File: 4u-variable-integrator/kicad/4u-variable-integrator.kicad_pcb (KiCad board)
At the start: 2 copper layers, 99.1 x 152.4 mm, 91 parts, among them J1 Banana Socket PanelMount, J10 Banana Socket PanelMount, J11 Banana Socket PanelMount, J12 Conn_01x04_Female, J13 Conn_01x04_Male, J14 Conn_01x02_Female, J15 Conn_01x02_Male, J16 Banana Socket PanelMount, J17 4U_Power, J18 Banana Socket PanelMount, J19 Banana Socket PanelMount, J2 Banana Socket PanelMount, J20 Conn_01x04_Female, J21 Conn_01x04_Male, J22 Banana Socket PanelMount, J23 Banana Socket PanelMount, J3 Banana Socket PanelMount, J4 Conn_01x04_Female, J5 Conn_01x04_Female, J6 Conn_01x04_Male, J7 Conn_01x04_Male, J8 Banana Socket PanelMount, J9 Banana Socket PanelMount, Q1 2N3906, Q2 2N3906, U1 TL074, U2 LM13700, U4 TL072

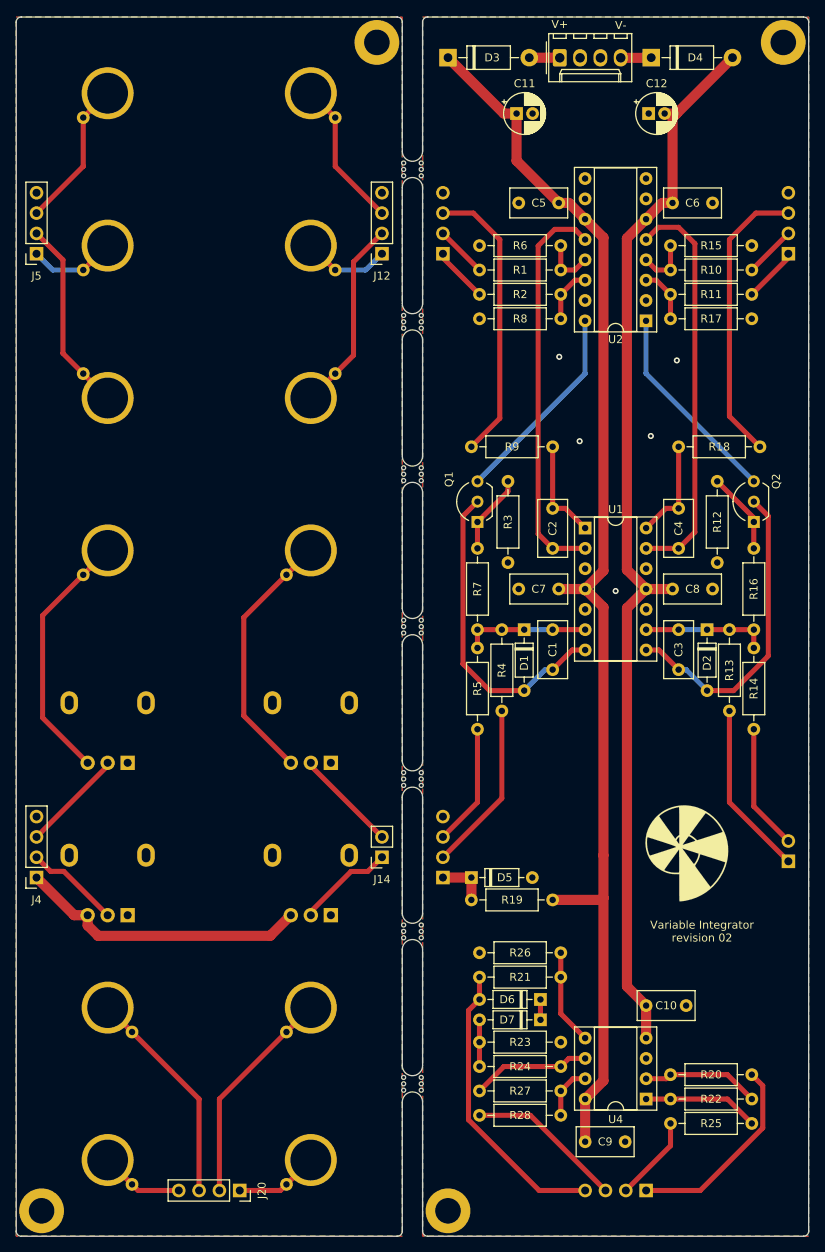
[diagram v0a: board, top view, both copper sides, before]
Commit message: Refreshing kicad projects
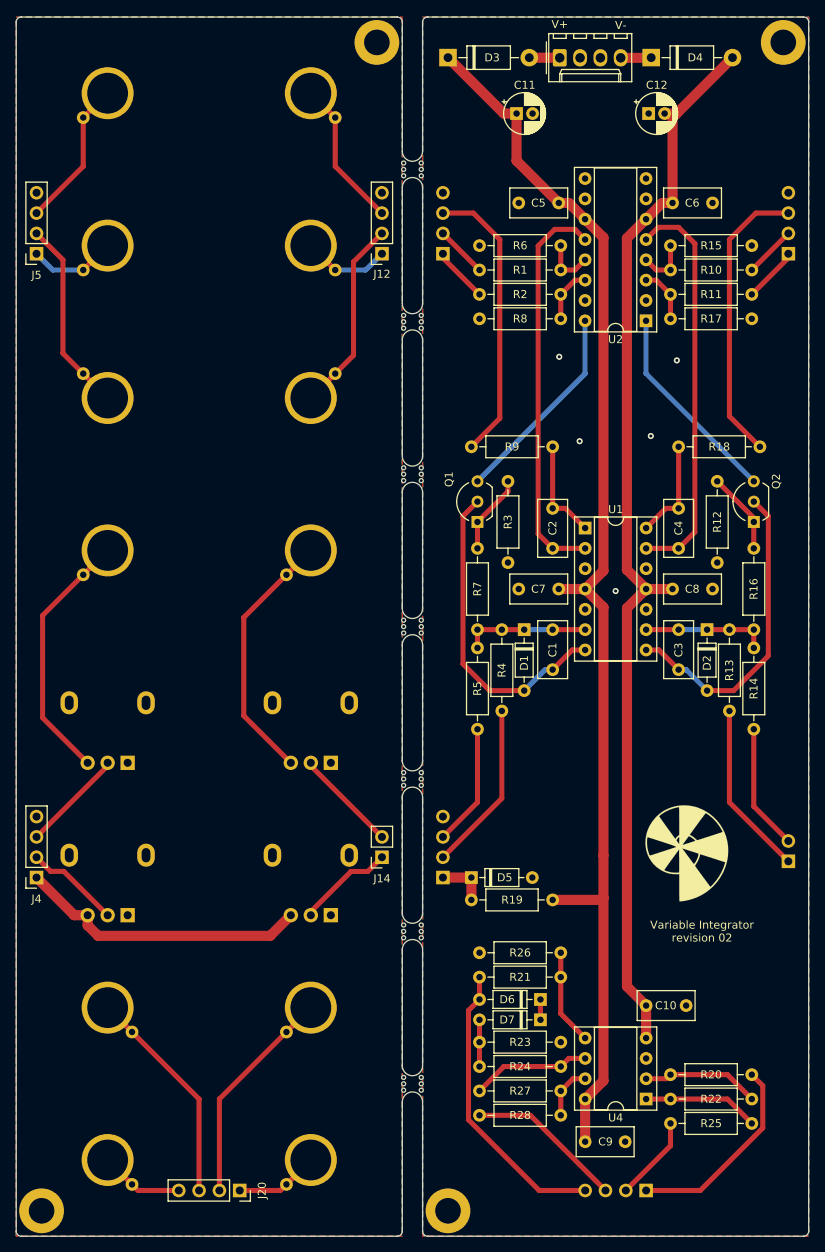
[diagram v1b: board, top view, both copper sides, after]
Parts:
- C1, C10, C2, C3, C4, C5, C6, C7, C8, C9: footprint rumblesan-standard-parts:C_Rect_L7.0mm_W3.5mm_P5.00mm -> Rumblesan_Standard_Parts:C_Rect_L7.0mm_W3.5mm_P5.00mm
- C11, C12: value 1uF -> 10uF; footprint rumblesan-standard-parts:CP_Radial_D5.0mm_P2.00mm -> Rumblesan_Standard_Parts:CP_Radial_D5.0mm_P2.00mm
- D1, D2: value 1n4148 -> 1N4148; footprint rumblesan-standard-parts:D_DO-35_SOD27_P7.62mm_Horizontal -> Rumblesan_Standard_Parts:D_DO-35_SOD27_P7.62mm_Horizontal
- D3, D4: footprint rumblesan-standard-parts:D_DO-41_SOD81_P10.16mm_Horizontal -> Rumblesan_Standard_Parts:D_DO-41_SOD81_P10.16mm_Horizontal
- D5, D6, D7: footprint rumblesan-standard-parts:D_DO-35_SOD27_P7.62mm_Horizontal -> Rumblesan_Standard_Parts:D_DO-35_SOD27_P7.62mm_Horizontal
- H1, H2, H3, H4: footprint rumblesan-standard-parts:MountingHole_3.2mm_M3_DIN965_Pad -> Rumblesan_Standard_Parts:MountingHole_3.2mm_M3_DIN965_Pad
- J1, J10, J11, J16, J18, J19, J2, J22, J23, J3, J8, J9: footprint rumblesan-standard-parts:BananaJack_THT_JohnsonCinch_108-09 -> Rumblesan_Standard_Parts:BananaJack_THT_JohnsonCinch_108-09
- J17: footprint 4u-power:4u_Power_Molex_KK-254_P2.54mm -> 4U_Power:4u_Power_Molex_KK-254_P2.54mm
- R1, R10, R11, R12, R13, R14, R15, R16, R17, R18, R19, R2, R20, R21, R22, R23, R24, R25, R26, R27, R28, R3, R4, R5, R6, R7, R8, R9: footprint rumblesan-standard-parts:R_Axial_DIN0207_L6.3mm_D2.5mm_P10.16mm_Horizontal -> Rumblesan_Standard_Parts:R_Axial_DIN0207_L6.3mm_D2.5mm_P10.16mm_Horizontal
- RV1, RV2, RV3, RV4: footprint rumblesan-standard-parts:Potentiometer_Alpha_RD901F-40-00D_Single_Vertical -> Rumblesan_Standard_Parts:Potentiometer_Alpha_RD901F-40-00D_Single_Vertical
- U1: footprint rumblesan-standard-parts:DIP-14_W7.62mm_Socket -> Rumblesan_Standard_Parts:DIP-14_W7.62mm_Socket
- U2: footprint rumblesan-standard-parts:DIP-16_W7.62mm_Socket -> Rumblesan_Standard_Parts:DIP-16_W7.62mm_Socket
- U4: footprint rumblesan-standard-parts:DIP-8_W7.62mm_Socket -> Rumblesan_Standard_Parts:DIP-8_W7.62mm_Socket
